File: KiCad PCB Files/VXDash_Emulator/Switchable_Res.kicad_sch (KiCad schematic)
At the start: 4 parts, among them Q4 2N7002

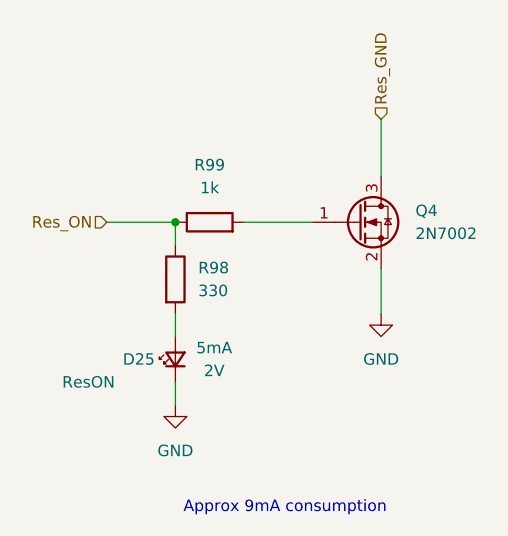
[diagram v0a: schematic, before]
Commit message: Emulator board : BOM and fab prep
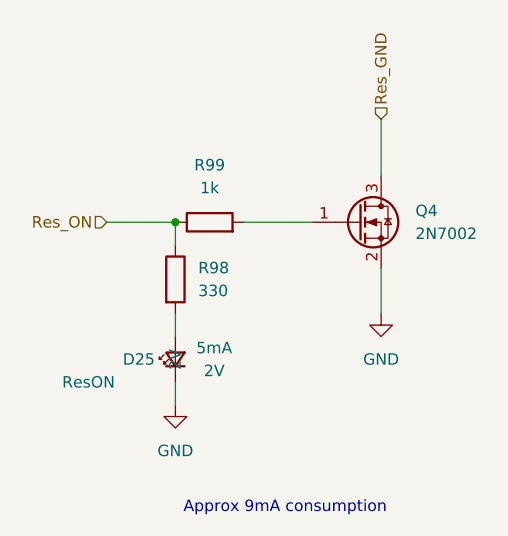
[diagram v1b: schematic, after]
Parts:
- D25: MFT (none) -> Harvatek Corp; MFT_PN (none) -> B1911UD--20D001014U1930; Voltage (none) -> 2V
- R98: MFT (none) -> Yageo; MFT_PN (none) -> RC0603FR-07330RL
- R99: MFT (none) -> Yageo; MFT_PN (none) -> RC0603FR-071KL
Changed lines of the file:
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@@
 			)
 		)
-		(property "Description" ""
+		(property "Description" "RES 330 OHM 1% 1/10W 0603"
 			(at 124.46 96.52 0)
 			(effects
@@
 			)
 		)
-		(property "MFT" ""
+		(property "MFT" "Yageo"
 			(at 124.46 96.52 0)
 			(effects
@@
 			)
 		)
-		(property "MFT_PN" ""
+		(property "MFT_PN" "RC0603FR-07330RL"
 			(at 124.46 96.52 0)
 			(effects
@@
 			)
 		)
-		(property "Description" ""
+		(property "Description" "RES 1K OHM 1% 1/10W 0603"
 			(at 128.27 90.17 0)
 			(effects
@@
 			)
 		)
-		(property "MFT" ""
-			(at 128.27 90.17 0)
-			(effects
-				(font
-					(size 1.27 1.27)
-				)
-				(hide yes)
-			)
-		)
-		(property "MFT_PN" ""
+		(property "MFT" "Yageo"
+			(at 128.27 90.17 0)
+			(effects
+				(font
+					(size 1.27 1.27)
+				)
+				(hide yes)
+			)
+		)
+		(property "MFT_PN" "RC0603FR-071KL"
 			(at 128.27 90.17 0)
 			(effects
@@
 			)
 		)
-		(property "Description" "Light emitting diode, small symbol"
+		(property "Description" "LED ORANGE DIFFUSED 0603 SMD"
 			(at 124.46 105.41 0)
 			(effects
@@
 			)
 		)
-		(property "MFT" ""
+		(property "MFT" "Harvatek Corp"
 			(at 124.46 105.41 0)
 			(effects
@@
 			)
 		)
-		(property "MFT_PN" ""
+		(property "MFT_PN" "B1911UD--20D001014U1930"
 			(at 124.46 105.41 0)
 			(effects
@@
 			(effects
 				(font
+					(size 1.27 1.27)
+				)
+			)
+		)
+		(property "Voltage" "2V"
+			(at 124.46 105.41 0)
+			(effects
+				(font

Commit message: Emulator : LCSC part numbers and production files
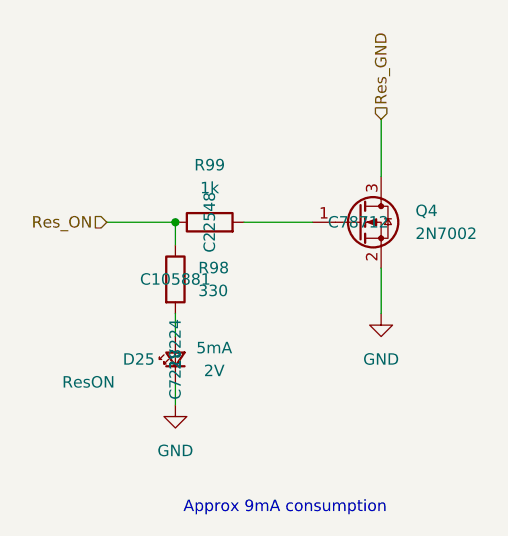
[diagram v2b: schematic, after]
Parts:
- D25: LCSC (none) -> C7218224
- Q4: LCSC (none) -> C78712
- R98: LCSC (none) -> C105881
- R99: LCSC (none) -> C22548
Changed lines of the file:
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@@
+			)
+		)
+		(property "LCSC" "C78712"
+			(at 144.78 90.17 0)
+			(effects
+				(font
+					(size 1.27 1.27)
+				)
 			)
 		)
@@
 			)
 		)
+		(property "LCSC" "C105881"
+			(at 124.46 96.52 0)
+			(effects
+				(font
+					(size 1.27 1.27)
+				)
+			)
+		)
 		(pin "1"
 		)
@@
 			)
 		)
+		(property "LCSC" "C22548"
+			(at 128.27 90.17 0)
+			(effects
+				(font
+					(size 1.27 1.27)
+				)
+			)
+		)
 		(pin "1"
 		)
@@
 			(at 124.46 105.41 0)
 			(effects
+				(font
+					(size 1.27 1.27)
+				)
+			)
+		)
+		(property "LCSC" "C7218224"
+			(at 124.46 105.41 0)
+			(effects

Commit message: Emulator : Updating BOM with LCSC alts
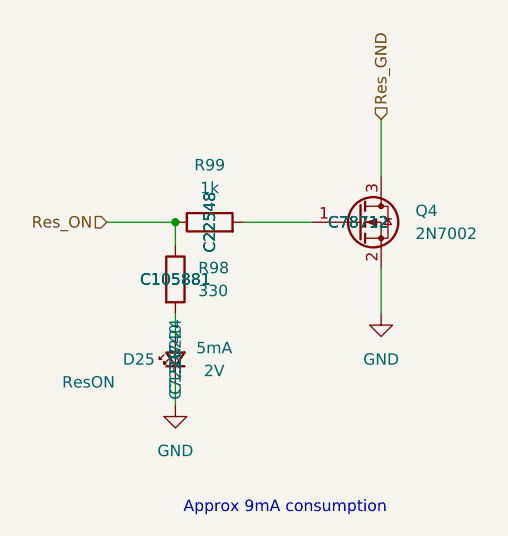
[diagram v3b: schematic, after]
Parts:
- D25: LCSC alt (none) -> C157740
- Q4: LCSC alt (none) -> C78712
- R98: LCSC alt (none) -> C105881
- R99: LCSC alt (none) -> C22548
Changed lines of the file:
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@@
+			)
+		)
+		(property "LCSC alt" "C78712"
+			(at 144.78 90.17 0)
+			(effects
+				(font
+					(size 1.27 1.27)
+				)
 			)
 		)
@@
 			)
 		)
+		(property "LCSC alt" "C105881"
+			(at 124.46 96.52 0)
+			(effects
+				(font
+					(size 1.27 1.27)
+				)
+			)
+		)
 		(pin "1"
 		)
@@
 			)
 		)
+		(property "LCSC alt" "C22548"
+			(at 128.27 90.17 0)
+			(effects
+				(font
+					(size 1.27 1.27)
+				)
+			)
+		)
 		(pin "1"
 		)
@@
 			(at 124.46 105.41 0)
 			(effects
+				(font
+					(size 1.27 1.27)
+				)
+			)
+		)
+		(property "LCSC alt" "C157740"
+			(at 124.46 105.41 0)
+			(effects
